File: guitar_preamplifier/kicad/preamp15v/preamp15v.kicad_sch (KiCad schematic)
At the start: 58 parts, among them J1 J201, P1A {P1a}, P1B {P1b}, P2A {P2a}, P2B {P2b}, P3A {P3a}, P3B {P3b}, P4B {P4b}, Q1 BC546B, Q2 BC556B, Q3 BC546B, Q4 BC546B, T20 560, T5 22k

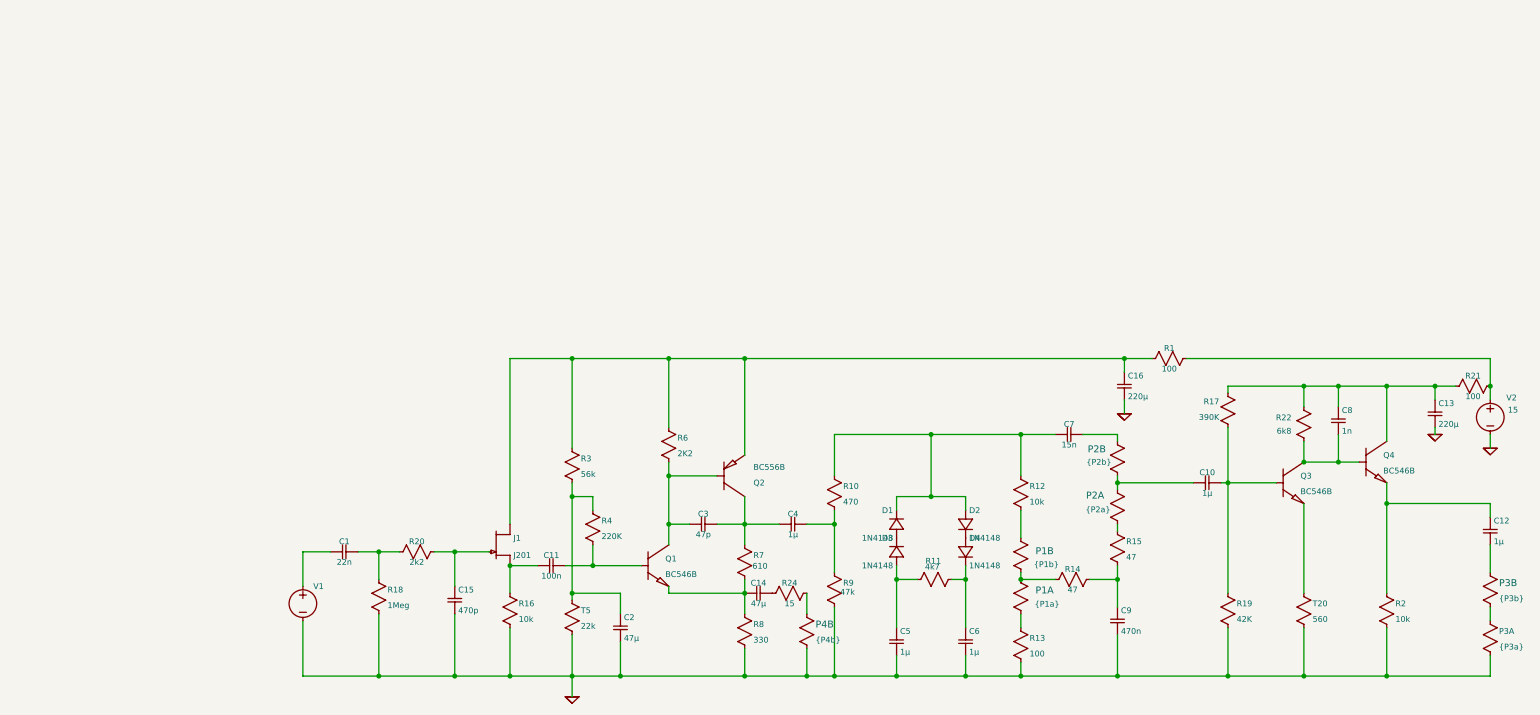
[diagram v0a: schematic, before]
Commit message: Update preamp15v
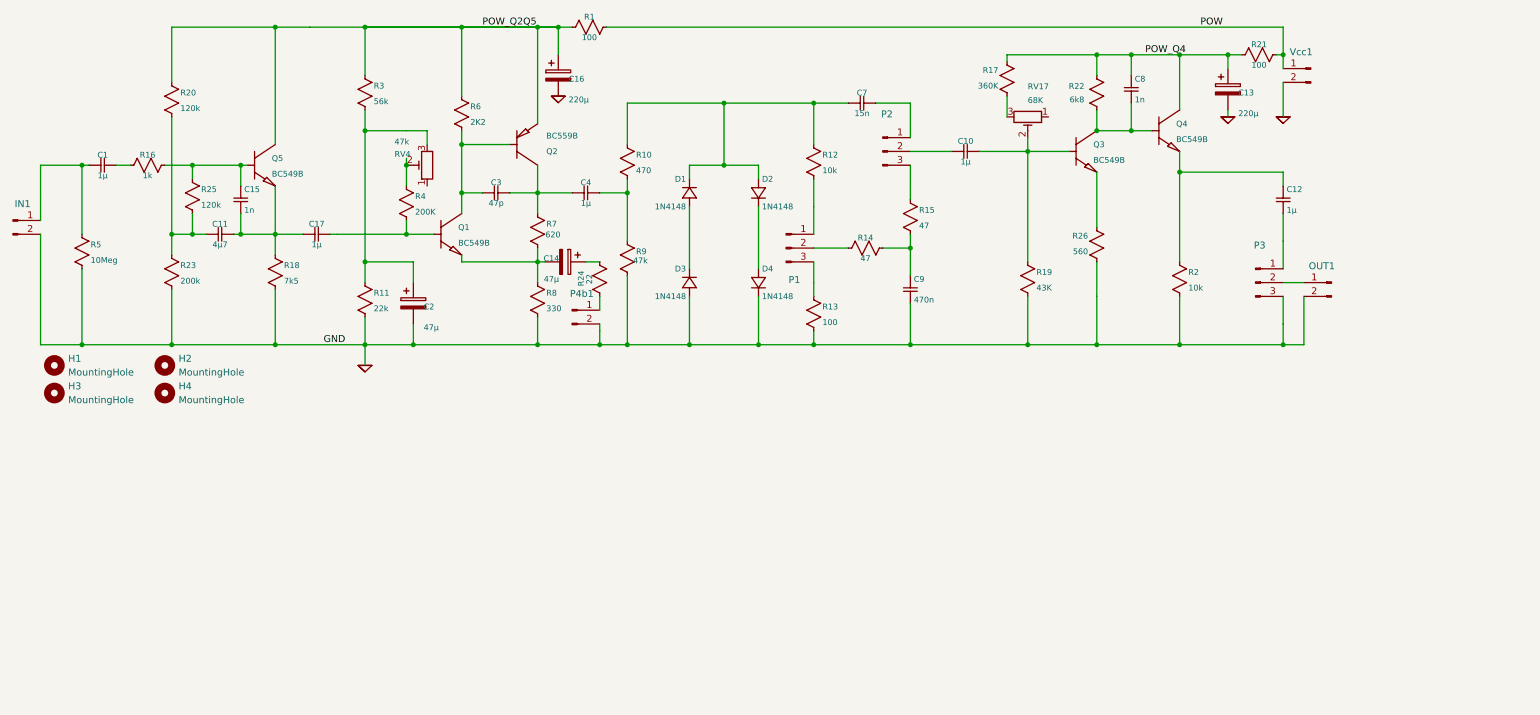
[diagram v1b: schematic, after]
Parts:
- removed C13, C16: 220µ, symbol ltspice:Cap
- removed C14, C2: 47µ, symbol ltspice:Cap
- removed C5, C6: 1µ, symbol ltspice:Cap
- removed J1: J201, symbol ltspice:njf
- removed P1A: {P1a}, symbol ltspice:Res
- removed P1B: {P1b}, symbol ltspice:Res
- removed P2A: {P2a}, symbol ltspice:Res
- removed P2B: {P2b}, symbol ltspice:Res
- removed P3A: {P3a}, symbol ltspice:Res
- removed P3B: {P3b}, symbol ltspice:Res
- removed P4B: {P4b}, symbol ltspice:Res
- removed T20: 560, symbol ltspice:Res
- removed T5: 22k, symbol ltspice:Res
- removed V1: SINE(0 {in_amplitude} {in_freq}), symbol ltspice:Voltage
- removed V2: 15, symbol ltspice:voltage
- added C13, C16: 220µ, electrucio_cnc_footprints:CP_Radial_220u_8mm_3.5mm_largerpads, symbol Device:C_Polarized
- added C14, C2: 47µ, electrucio_cnc_footprints:CP_Radial_D5.0mm_P2.00mm_largerpads, symbol Device:C_Polarized
- added C17: 1µ, electrucio_cnc_footprints:C_Rect_WIMA_1uF_CNC_LargePads, symbol ltspice:Cap
- added H1, H2, H3, H4: MountingHole, MountingHole:MountingHole_3.5mm, symbol Mechanical:MountingHole
- added IN1, OUT1, P4b1, Vcc1: (no value), electrucio_cnc_footprints:JST_XH_B2B-XH-A_1x02_P2.50mm_Vertical_ovalpads, symbol Connector:Conn_01x02_Pin
- added P1, P2, P3: (no value), electrucio_cnc_footprints:JST_XH_B3B-XH-A_1x03_P2.50mm_Vertical_ovalpads, symbol Connector:Conn_01x03_Pin
- added Q5: BC549B, electrucio_cnc_footprints:TO-92_Inline_Wide_largerpads, symbol ltspice:npn
- added R23: 200k, electrucio_cnc_footprints:R_Axial_DIN0207_L6.3mm_D2.5mm_P10.16mm_Horizontal_LargerPads, symbol ltspice:Res
- added R25: 120k, electrucio_cnc_footprints:R_Axial_DIN0207_L6.3mm_D2.5mm_P10.16mm_Horizontal_LargerPads, symbol ltspice:Res
- added R26: 560, electrucio_cnc_footprints:R_Axial_DIN0207_L6.3mm_D2.5mm_P10.16mm_Horizontal_LargerPads, symbol ltspice:Res
- added R5: 10Meg, electrucio_cnc_footprints:R_Axial_DIN0207_L6.3mm_D2.5mm_P10.16mm_Horizontal_LargerPads, symbol ltspice:Res
- added RV17: 68K, electrucio_cnc_footprints:Potentiometer_Piher_PT-6-V_Vertical_largerpads, symbol Device:R_Potentiometer_Trim
- added RV4: 47k, electrucio_cnc_footprints:Potentiometer_Piher_PT-6-V_Vertical_largerpads, symbol Device:R_Potentiometer_Trim
- C1: value 22n -> 1µ; footprint (none) -> electrucio_cnc_footprints:C_Rect_WIMA_1uF_CNC_LargePads
- C10, C12, C4, C8: footprint (none) -> electrucio_cnc_footprints:C_Rect_WIMA_1uF_CNC_LargePads
- C11: value 100n -> 4µ7; footprint (none) -> electrucio_cnc_footprints:CP_Radial_D5.0mm_P2.00mm_largerpads
- C15: value 470p -> 1n; footprint (none) -> electrucio_cnc_footprints:C_Rect_WIMA_1uF_CNC_LargePads
- C3: footprint (none) -> electrucio_cnc_footprints:C_Disc_D4.3mm_W1.9mm_P5.00mm_largerpads
- C7: footprint (none) -> Capacitor_THT:C_Rect_L13.0mm_W4.0mm_P10.00mm_FKS3_FKP3_MKS4
- C9: footprint (none) -> Capacitor_THT:C_Rect_L26.5mm_W10.5mm_P22.50mm_MKS4
- D1, D2, D3, D4: footprint (none) -> electrucio_cnc_footprints:D_DO-35_SOD27_P7.62mm_Horizontal_largerpads
- Q1, Q3, Q4: value BC546B -> BC549B; footprint (none) -> electrucio_cnc_footprints:TO-92_Inline_Wide_largerpads
- Q2: value BC556B -> BC559B; footprint (none) -> electrucio_cnc_footprints:TO-92_Inline_Wide_largerpads
- R1, R10, R12, R13, R15, R2, R21, R22, R3, R6, R8, R9: footprint R_Axial_DIN0207_L6.3mm_D2.5mm_P10.16mm_Horizontal -> electrucio_cnc_footprints:R_Axial_DIN0207_L6.3mm_D2.5mm_P10.16mm_Horizontal_LargerPads
- R11: value 4k7 -> 22k; footprint R_Axial_DIN0207_L6.3mm_D2.5mm_P10.16mm_Horizontal -> electrucio_cnc_footprints:R_Axial_DIN0207_L6.3mm_D2.5mm_P10.16mm_Horizontal_LargerPads
- R14: footprint (none) -> electrucio_cnc_footprints:R_Axial_DIN0207_L6.3mm_D2.5mm_P10.16mm_Horizontal_LargerPads
- R16: value 10k -> 1k; footprint R_Axial_DIN0207_L6.3mm_D2.5mm_P10.16mm_Horizontal -> electrucio_cnc_footprints:R_Axial_DIN0207_L6.3mm_D2.5mm_P10.16mm_Horizontal_LargerPads
- R17: value 390K -> 360K; footprint R_Axial_DIN0207_L6.3mm_D2.5mm_P10.16mm_Horizontal -> electrucio_cnc_footprints:R_Axial_DIN0207_L6.3mm_D2.5mm_P10.16mm_Horizontal_LargerPads
- R18: value 1Meg -> 7k5; footprint Resistor_THT:R_Axial_DIN0207_L6.3mm_D2.5mm_P10.16mm_Horizontal -> electrucio_cnc_footprints:R_Axial_DIN0207_L6.3mm_D2.5mm_P10.16mm_Horizontal_LargerPads
- R19: value 42K -> 43K; footprint R_Axial_DIN0207_L6.3mm_D2.5mm_P10.16mm_Horizontal -> electrucio_cnc_footprints:R_Axial_DIN0207_L6.3mm_D2.5mm_P10.16mm_Horizontal_LargerPads
- R20: value 2k2 -> 120k; footprint R_Axial_DIN0207_L6.3mm_D2.5mm_P10.16mm_Horizontal -> electrucio_cnc_footprints:R_Axial_DIN0207_L6.3mm_D2.5mm_P10.16mm_Horizontal_LargerPads
- R24: value 15 -> 22; footprint R_Axial_DIN0207_L6.3mm_D2.5mm_P10.16mm_Horizontal -> electrucio_cnc_footprints:R_Axial_DIN0207_L6.3mm_D2.5mm_P10.16mm_Horizontal_LargerPads
- R4: value 220K -> 200K; footprint R_Axial_DIN0207_L6.3mm_D2.5mm_P10.16mm_Horizontal -> electrucio_cnc_footprints:R_Axial_DIN0207_L6.3mm_D2.5mm_P10.16mm_Horizontal_LargerPads
- R7: value 610 -> 620; footprint R_Axial_DIN0207_L6.3mm_D2.5mm_P10.16mm_Horizontal -> electrucio_cnc_footprints:R_Axial_DIN0207_L6.3mm_D2.5mm_P10.16mm_Horizontal_LargerPads
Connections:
- net 0: now also D3.1 (+), D4.2 (-), R11.2, C13.2, C16.2, C2.2, IN1.2 (Pin_2), OUT1.2 (Pin_2), P3.3 (Pin_3), P4b1.2 (Pin_2), R23.2, R26.1, R5.2, Vcc1.2 (Pin_2); no longer C15.2, R16.2
- net POW_Q2Q5: now reaches Q2.3 (E), R1.2, R3.1, R6.1
- net POW_Q2Q5: now also R20.1, C16.1, Q5.1 (C)
- net at C15.1: now also R16.1, Q5.2 (B), R25.1; no longer R20.1
- net at C11.2: now also R20.2, R23.1, R25.2; no longer R16.1
- net POW_Q4: now reaches C8.1, Q4.1 (C), R17.2, R21.2, R22.1
- net POW_Q4: now also C13.1
- net at R12.2: now also P1.1 (Pin_1)
- net at C10.1, Q3.2 (B), R19.1: now also RV17.2; no longer R17.1
- net at C10.2: now also P2.2 (Pin_2)
- net POW: now reaches R1.1, R21.1
- net POW: now also Vcc1.1 (Pin_1)
- net at R11.1: now also R3.2, C2.1, RV4.3; no longer D4.2 (-)
- net at C12.2: now also P3.1 (Pin_1)
- net at R4.1: now also RV4.2; no longer R3.2
- net at R15.1: now also P2.3 (Pin_3)
- net at R24.1: now also P4b1.1 (Pin_1)
- net at C1.2: now also IN1.1 (Pin_1), R5.1
- net at R24.2: now also C14.1
- net at Q1.3 (E), R7.2, R8.1: now also C14.2
- net at C7.1: now also P2.1 (Pin_1)
- net at R14.2: now also P1.2 (Pin_2)
- net at R13.1: now also P1.3 (Pin_3)
- net at Q1.2 (B), R4.2: now also C17.1; no longer C11.1
- net at Q3.3 (E): now also R26.2
- new net: C11.1, C15.2, C17.2, Q5.3 (E), R18.1
- new net: C1.1, R16.2
- new net: R17.1, RV17.3
- new net: OUT1.1 (Pin_1), P3.2 (Pin_2)
